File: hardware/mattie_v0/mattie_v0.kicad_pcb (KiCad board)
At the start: 4 copper layers, 55 x 32 mm, 52 parts, among them J1 5V, J2 USB_B_Mini, J3 Power, U1 STM32F40X_LQFP64, U2 ICE40UP5K-SG48ITR, U3 MCP1826T, U4 MCP1826S-3302, U5 DSC1004, Y1 8Mhz

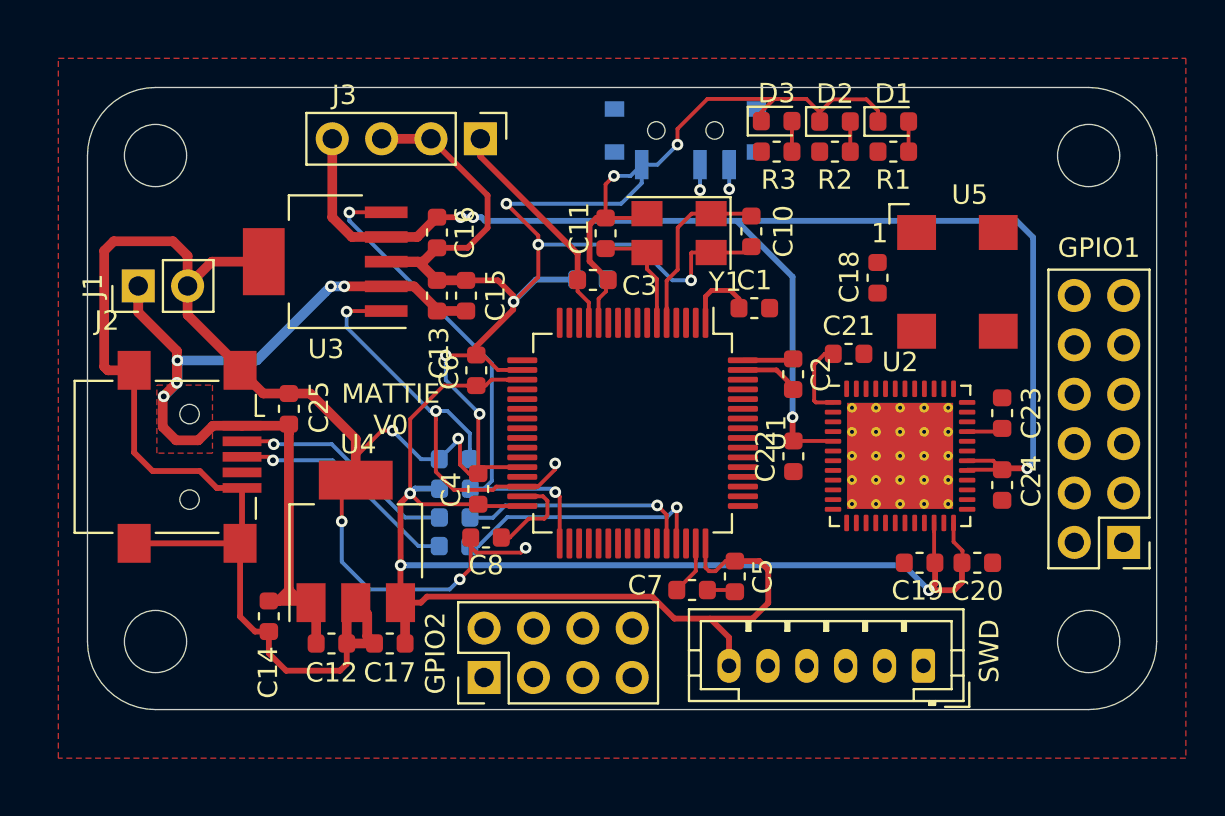
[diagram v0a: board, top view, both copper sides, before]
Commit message: routing
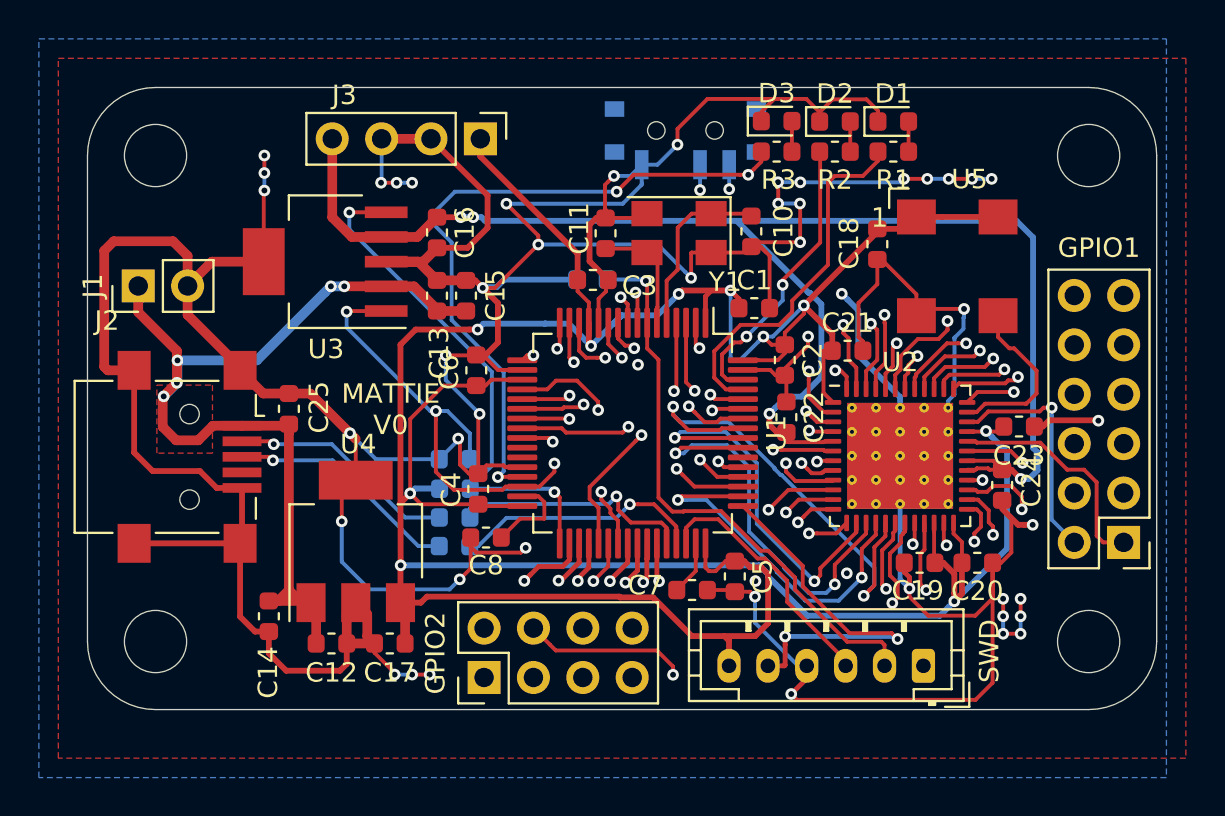
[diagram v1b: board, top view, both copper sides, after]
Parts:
- moved C22 2.04 mm to (163.4, 133.5), turned to 270 degrees
- moved C18 1.73 mm to (168.1, 124.6)
- moved C23 1.11 mm to (175.4, 133.9), turned to 0 degrees
- moved C2 0.85 mm to (163.4, 130.5)
- moved U5 0.80 mm to (172.2, 125.7)
- moved C21 0.17 mm to (166.6, 130.0)
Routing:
- net GND: track 203.5 -> 363.8 mm, vias 13 -> 46
- net +3V3: track 118.0 -> 194.3 mm, vias 4 -> 11
- net /LATTICE_ICE40/DAT5: track 0.00 -> 35.1 mm, vias 0 -> 2
- net /MCU/LED_RED: track 0.00 -> 35.0 mm, vias 0 -> 3
- net /LATTICE_ICE40/DAT14: track 0.00 -> 32.9 mm, vias 0 -> 2
- net /MCU/NRST: track 0.00 -> 29.7 mm, vias 0 -> 1
- net /LATTICE_ICE40/DAT12: track 0.00 -> 29.0 mm, vias 0 -> 2
- net /LATTICE_ICE40/DAT15: track 0.00 -> 28.8 mm, vias 0 -> 2
- net /LATTICE_ICE40/DAT13: track 0.00 -> 28.3 mm, vias 0 -> 2
- net /LATTICE_ICE40/AUX2: track 0.00 -> 28.2 mm, vias 0 -> 3
- net /LATTICE_ICE40/DAT7: track 0.00 -> 26.9 mm, vias 0 -> 2
- net /LATTICE_ICE40/AUX5: track 0.00 -> 26.8 mm, vias 0 -> 2
- net /LATTICE_ICE40/AUX4: track 0.00 -> 25.6 mm, vias 0 -> 3
- net /LATTICE_ICE40/SPI_MOSI: track 0.00 -> 24.3 mm, vias 0 -> 2
- net /LATTICE_ICE40/DAT4: track 0.00 -> 23.8 mm, vias 0 -> 2
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- added copper zone on B.Cu, net GND
- added copper zone on In1.Cu, net GND
- added copper zone on In2.Cu, net GND

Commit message: tweaking and cleaning
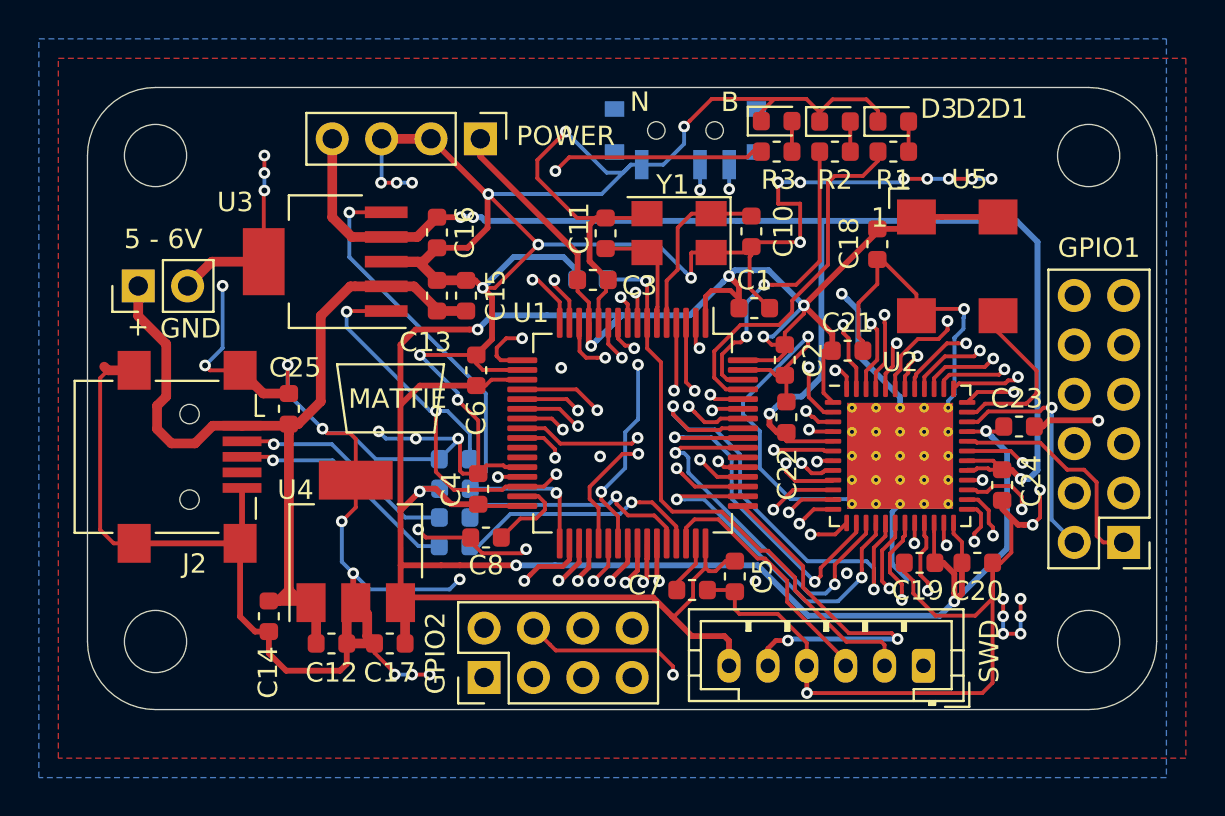
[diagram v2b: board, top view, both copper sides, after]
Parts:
- 5 - 6V: renamed from J1
- renumbered J3 to POWER
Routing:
- net GND: track 363.8 -> 399.6 mm, vias 46 -> 52
- net +3V3: track 194.3 -> 188.2 mm, vias 11 -> 10
- net /LATTICE_ICE40/DAT2: track 21.8 -> 26.7 mm
- net /LATTICE_ICE40/DAT1: track 18.2 -> 22.8 mm
- net /DCDC/5V: track 50.3 -> 46.5 mm, vias 5 -> 0
- net /LATTICE_ICE40/DAT3: track 21.9 -> 25.5 mm
- net /LATTICE_ICE40/SPI_SCK: track 21.1 -> 19.3 mm
- net +1V2: track 77.4 -> 75.5 mm
- net /LATTICE_ICE40/DAT6: track 23.5 -> 21.9 mm
- net /LATTICE_ICE40/DAT14: track 32.9 -> 31.7 mm
- net /LATTICE_ICE40/DAT4: track 23.8 -> 22.7 mm
- net /LATTICE_ICE40/DAT7: track 26.9 -> 25.9 mm
- net /MCU/LED_YELLOW: track 14.9 -> 15.9 mm
- net /LATTICE_ICE40/DAT12: track 29.0 -> 29.8 mm
- net /LATTICE_ICE40/SPI_MISO: track 19.7 -> 19.0 mm
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- removed copper zone on F.Cu, net /DCDC/5V
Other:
- board text added: "+"
- board text added: "B"
- board text added: "GND"
- board text added: "MATTIE"
- board text added: "N"
- board text removed: "MATTIE V0"
